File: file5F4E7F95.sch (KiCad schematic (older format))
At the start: 22 parts, among them U3 LTC7103

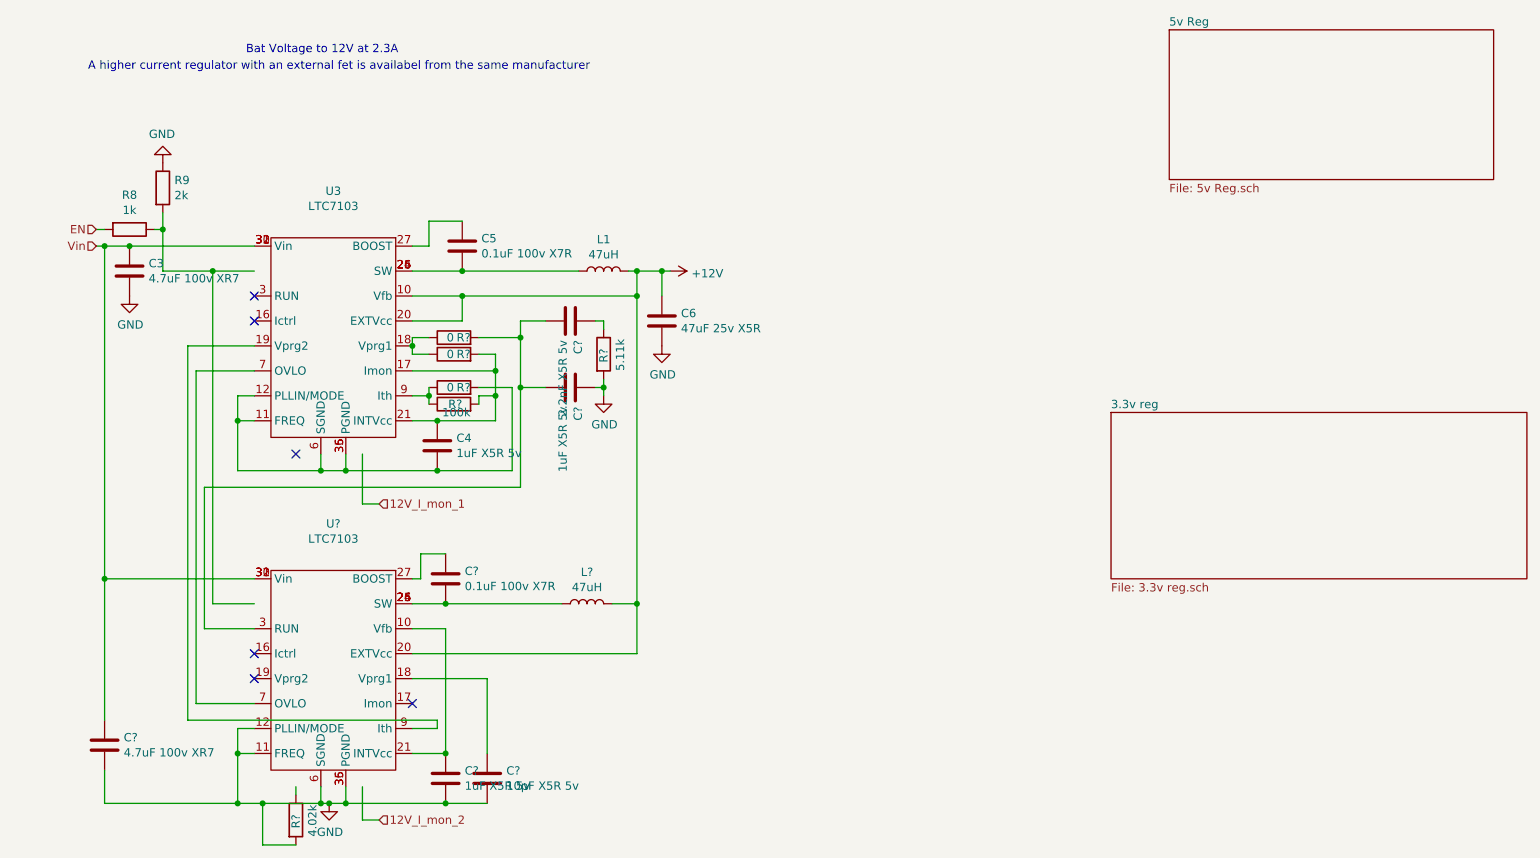
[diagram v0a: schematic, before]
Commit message: Revert "2 12v reg v"
This reverts commit 039d006401861a5917fcf1b07647dbdfad4f578a.
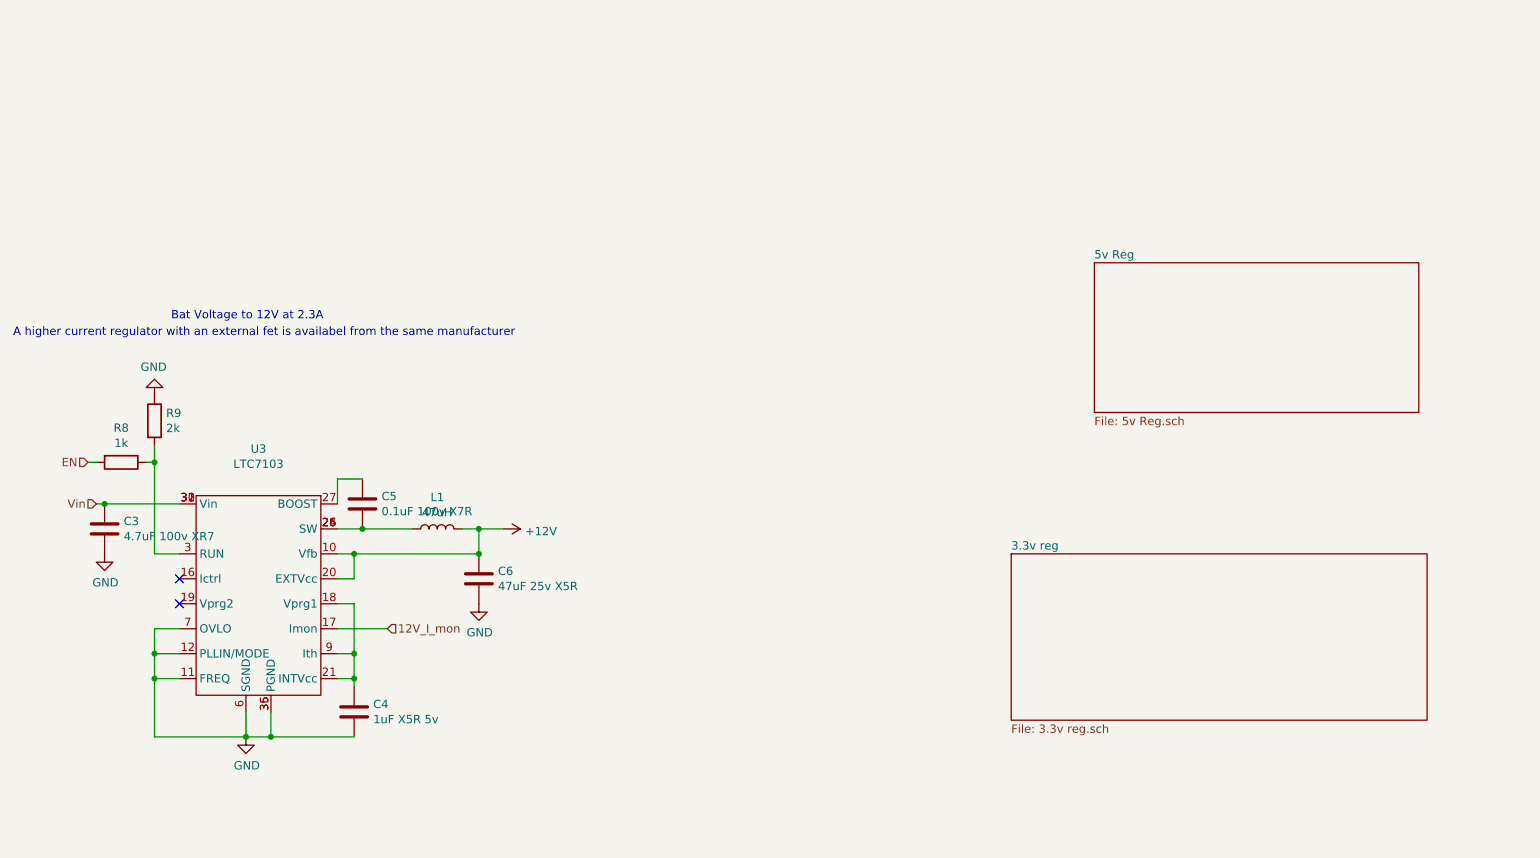
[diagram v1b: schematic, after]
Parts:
- removed C?: 4.7uF 100v XR7, Capacitor_SMD:C_0805_2012Metric, symbol Device:C
- removed C?: 2.2nF X5R 5v, Capacitor_SMD:C_0805_2012Metric, symbol Device:C
- removed C? (x2): 1uF X5R 5v, Capacitor_SMD:C_0805_2012Metric, symbol Device:C
- removed C?: 10pF X5R 5v, Capacitor_SMD:C_0805_2012Metric, symbol Device:C
- removed C?: 0.1uF 100v X7R, Capacitor_SMD:C_0805_2012Metric, symbol Device:C
- removed L?: 47uH, Inductor_SMD:L_Wuerth_WE-PD-Typ-LS, symbol Device:L
- removed R?: 100k, Resistor_SMD:R_0805_2012Metric, symbol Device:R
- removed R? (x3): 0, Resistor_SMD:R_0805_2012Metric, symbol Device:R
- removed R?: 5.11k, Resistor_SMD:R_0805_2012Metric, symbol Device:R
- removed R?: 4.02k, Resistor_SMD:R_0805_2012Metric, symbol Device:R
- removed U?: LTC7103, Package_DFN_QFN:QFN-36-1EP_5x6mm_P0.5mm_EP3.6x4.6mm_ThermalVias, symbol my_parts:LTC7103
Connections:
- net labels added: 12V_I_mon
- net labels removed: 12V_I_mon_1, 12V_I_mon_2
- wire segments 113 -> 36
- no-connect marks 6 -> 2
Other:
- moved on the sheet: C3, C4, C5, C6, L1, R8, R9, U3
